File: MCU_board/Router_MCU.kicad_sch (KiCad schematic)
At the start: 71 parts, among them J1 Header, T1 HY601742, U1 MYC-YT507H, U2 TPS54540, U3 LAN8720A, X1 B4B-XH, X2 B4B-XH, X3 B4B-XH, X4 B4B-XH, X5 B2B-XH, X6 TFP09-2-12B, X7 RJ45, Y1 25MHz

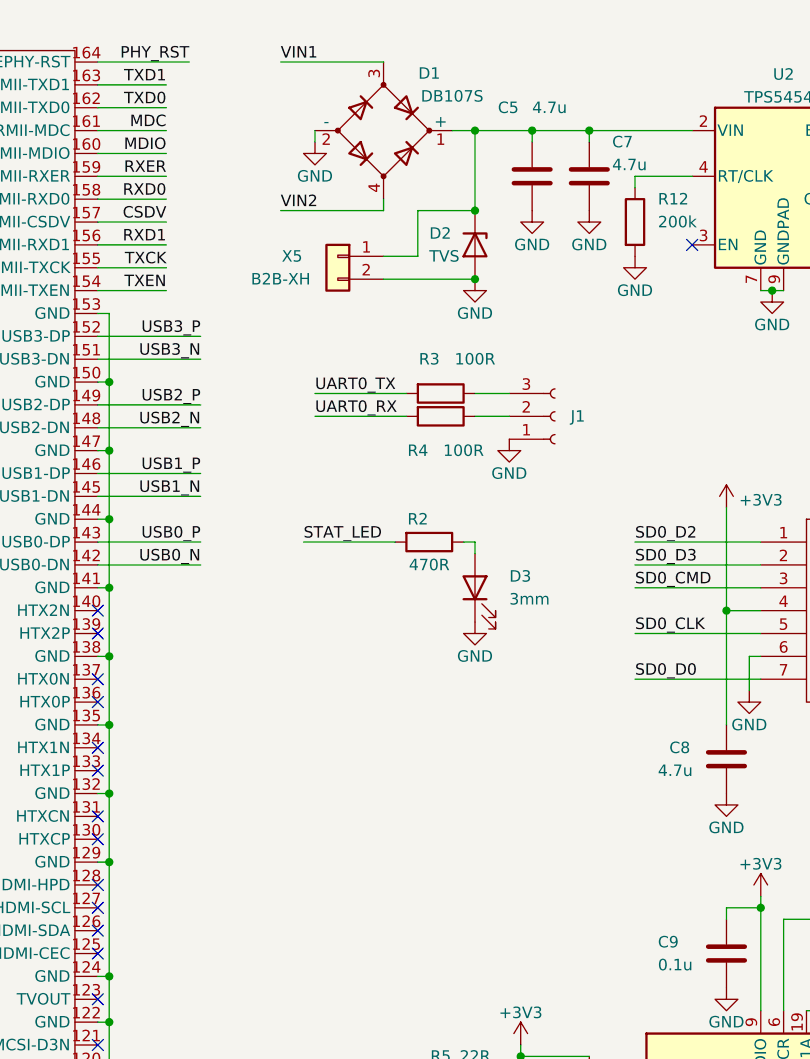
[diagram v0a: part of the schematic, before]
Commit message: Modems board ready
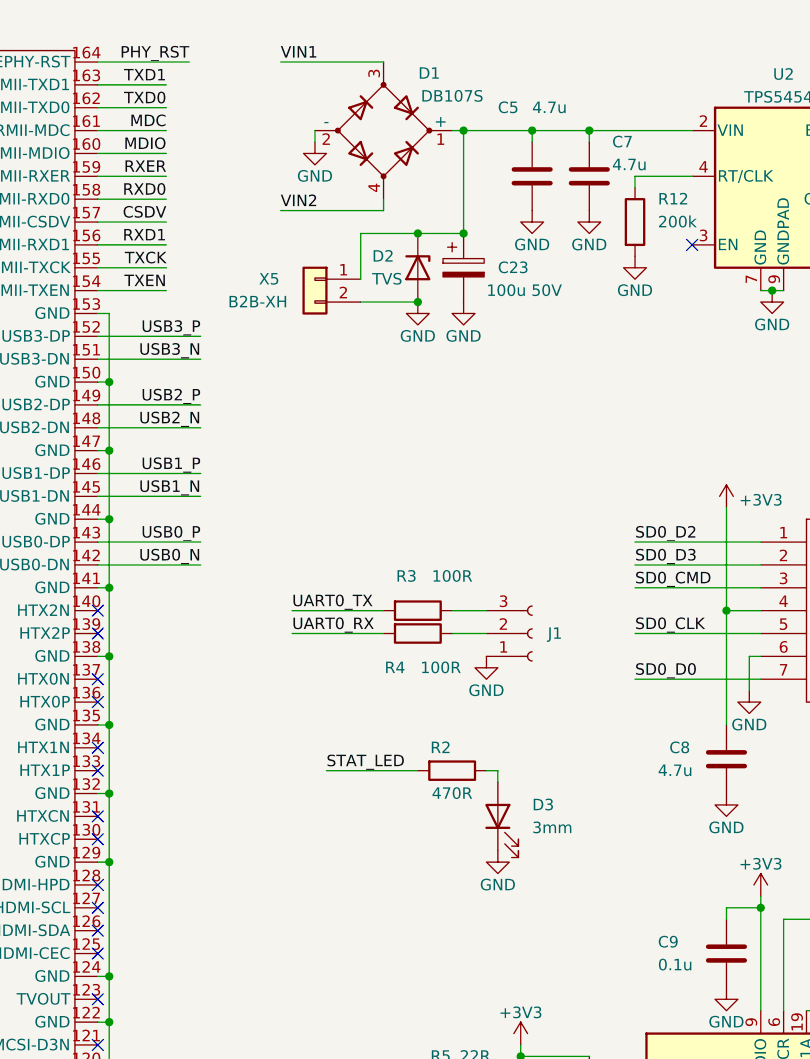
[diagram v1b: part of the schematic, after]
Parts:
- added C23: 100u 50V, Capacitor_SMD:CP_Elec_10x10.5, symbol Device:C_Polarized
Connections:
- net GND: now also C23.2
- net at C5.1, C7.1, D1.1 (+)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: now also C23.1
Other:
- moved on the sheet: D2, D3, J1, R2, R3, R4, X5
